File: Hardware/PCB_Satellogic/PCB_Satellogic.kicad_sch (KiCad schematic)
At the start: 4 parts, among them U1 E22-900M30S_LoRa, U2 Node-MCU_ESP32_38PINES, U3 TP4065_Modulo_cargador_de_bat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

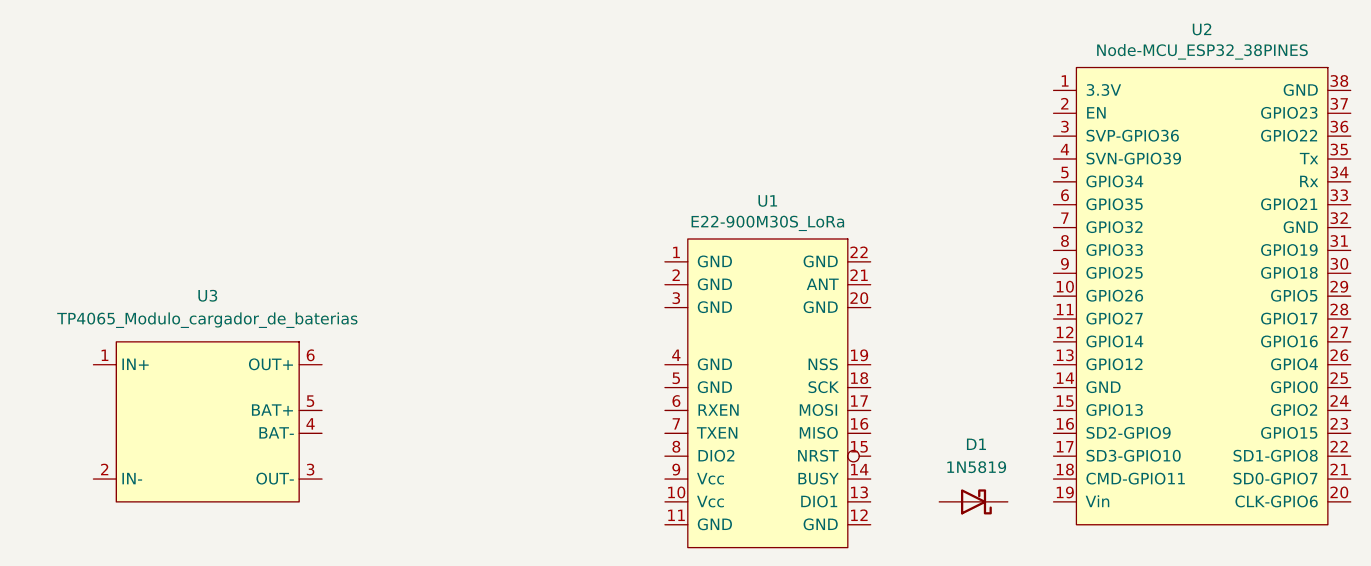
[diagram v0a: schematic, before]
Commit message: Introducción HW
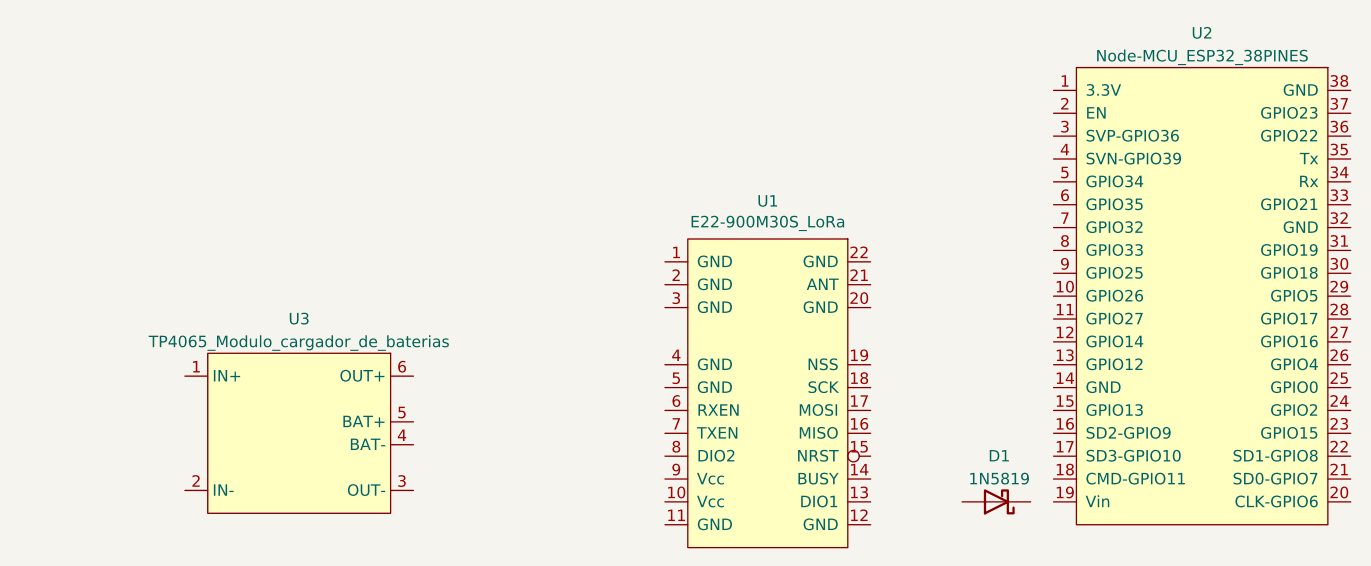
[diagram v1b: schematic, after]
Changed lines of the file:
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@@
-(kicad_sch (version 20211123) (generator eeschema)
+(kicad_sch (version 20230121) (generator eeschema)
   (paper "A4")
   (symbol (lib_id "Device:E22-900M30S_LoRa") (at 124.46 68.58 0) (unit 1)
-    (in_bom yes) (on_board yes)
-    (property "Reference" "U1" (id 0) (at 124.46 47.879 0))
-    (property "Value" "E22-900M30S_LoRa" (id 1) (at 124.46 50.1904 0))
-    (property "Footprint" "PCB_Satellogic:E22-900M30S_LoRa_smd" (id 2) (at 123.19 60.96 0)
+    (in_bom yes) (on_board yes) (dnp no)
+    (property "Reference" "U1" (at 124.46 47.879 0)
+      (effects (font (size 1.27 1.27)))
+    )
+    (property "Value" "E22-900M30S_LoRa" (at 124.46 50.1904 0)
+      (effects (font (size 1.27 1.27)))
+    )
+    (property "Footprint" "PCB_Satellogic:E22-900M30S_LoRa_smd" (at 123.19 60.96 0)
       (effects (font (size 1.27 1.27)) hide)
     )
-    (property "Datasheet" "" (id 3) (at 123.19 60.96 0)
+    (property "Datasheet" "" (at 123.19 60.96 0)
       (effects (font (size 1.27 1.27)) hide)
     )
@@
     (pin "8")
     (pin "9")
+    (instances
+      (project "PCB_Satellogic"
+        (path "/1c395ffa-f49b-425d-a435-d93dd675dfd0"
+          (reference "U1") (unit 1)
+        )
+      )
+    )
+  )
+  (symbol (lib_id "Diode:1N5819") (at 149.86 81.28 180) (unit 1)
+    (in_bom yes) (on_board yes) (dnp no) (fields_autoplaced)
+    (property "Reference" "D1" (at 150.1775 76.2 0)
+      (effects (font (size 1.27 1.27)))
+    )
+    (property "Value" "1N5819" (at 150.1775 78.74 0)
+      (effects (font (size 1.27 1.27)))
+    )
+    (property "Footprint" "Diode_THT:D_DO-41_SOD81_P10.16mm_Horizontal" (at 149.86 76.835 0)
+      (effects (font (size 1.27 1.27)) hide)
+    )
+    (property "Datasheet" "http://www.vishay.com/docs/88525/1n5817.pdf" (at 149.86 81.28 0)
+      (effects (font (size 1.27 1.27)) hide)
+    )
+    (pin "1")
+    (pin "2")
+    (instances
+      (project "PCB_Satellogic"
+        (path "/1c395ffa-f49b-425d-a435-d93dd675dfd0"
+          (reference "D1") (unit 1)
+        )
+      )
+    )
   )
   (symbol (lib_id "Device:Node-MCU_ESP32_38PINES") (at 172.72 57.15 0) (unit 1)
-    (in_bom yes) (on_board yes)
-    (property "Reference" "U2" (id 0) (at 172.72 28.829 0))
-    (property "Value" "Node-MCU_ESP32_38PINES" (id 1) (at 172.72 31.1404 0))
-    (property "Footprint" "PCB_Satellogic:Node-MCU_ESP32_38PINES_THT_offset" (id 2) (at 180.34 68.58 0)
+    (in_bom yes) (on_board yes) (dnp no) (fields_autoplaced)
+    (property "Reference" "U2" (at 172.72 29.21 0)
+      (effects (font (size 1.27 1.27)))
+    )
+    (property "Value" "Node-MCU_ESP32_38PINES" (at 172.72 31.75 0)
+      (effects (font (size 1.27 1.27)))
+    )
+    (property "Footprint" "PCB_Satellogic:Node-MCU_ESP32_38PINES_THT_offset" (at 180.34 68.58 0)
       (effects (font (size 1.27 1.27)) hide)
     )
-    (property "Datasheet" "" (id 3) (at 180.34 68.58 0)
+    (property "Datasheet" "" (at 180.34 68.58 0)
       (effects (font (size 1.27 1.27)) hide)
     )
@@
     (pin "8")
     (pin "9")
+    (instances
+      (project "PCB_Satellogic"
+        (path "/1c395ffa-f49b-425d-a435-d93dd675dfd0"
+          (reference "U2") (unit 1)
+        )
+      )
+    )
   )
-  (symbol (lib_id "Diode:1N5819") (at 147.32 81.28 180) (unit 1)
-    (in_bom yes) (on_board yes) (fields_autoplaced)
-    (property "Reference" "D1" (id 0) (at 147.6375 74.93 0))
-    (property "Value" "1N5819" (id 1) (at 147.6375 77.47 0))
-    (property "Footprint" "Diode_THT:D_DO-41_SOD81_P10.16mm_Horizontal" (id 2) (at 147.32 76.835 0)
+  (symbol (lib_id "Libreria_Proyecto_Satellogic:TP4065_Modulo_cargador_de_baterias") (at 72.39 73.66 0) (unit 1)
+    (in_bom yes) (on_board yes) (dnp no) (fields_autoplaced)
+    (property "Reference" "U3" (at 72.39 60.96 0)
+      (effects (font (size 1.27 1.27)))
+    )
+    (property "Value" "TP4065_Modulo_cargador_de_baterias" (at 72.39 63.5 0)
+      (effects (font (size 1.27 1.27)))
+    )
+    (property "Footprint" "PCB_Satellogic:TP4056" (at 71.12 68.58 0)
       (effects (font (size 1.27 1.27)) hide)
     )
-    (property "Datasheet" "http://www.vishay.com/docs/88525/1n5817.pdf" (id 3) (at 147.32 81.28 0)
-      (effects (font (size 1.27 1.27)) hide)
-    )
-    (pin "1")
-    (pin "2")
-  )
-  (symbol (lib_id "Libreria_Proyecto_Satellogic:TP4065_Modulo_cargador_de_baterias") (at 62.23 72.39 0) (unit 1)
-    (in_bom yes) (on_board yes) (fields_autoplaced)
-    (property "Reference" "U3" (id 0) (at 62.23 58.42 0))
-    (property "Value" "TP4065_Modulo_cargador_de_baterias" (id 1) (at 62.23 60.96 0))
-    (property "Footprint" "PCB_Satellogic:TP4056" (id 2) (at 60.96 67.31 0)
-      (effects (font (size 1.27 1.27)) hide)
-    )
-    (property "Datasheet" "" (id 3) (at 60.96 67.31 0)
+    (property "Datasheet" "" (at 71.12 68.58 0)
       (effects (font (size 1.27 1.27)) hide)
     )
@@
     (pin "5")
     (pin "6")
+    (instances
+      (project "PCB_Satellogic"
+        (path "/1c395ffa-f49b-425d-a435-d93dd675dfd0"
+          (reference "U3") (unit 1)
+        )
+      )
+    )
   )
   (sheet_instances
     (path "/" (page "1"))
   )
-  (symbol_instances
-    (path "/9dc25e6c-ccc6-4fa7-a0b9-7dc1baf8ff68"
-      (reference "D1") (unit 1) (value "1N5819") (footprint "Diode_THT:D_DO-41_SOD81_P10.16mm_Horizontal")
-    )
-    (path "/00000000-0000-0000-0000-0000640a4933"
-      (reference "U1") (unit 1) (value "E22-900M30S_LoRa") (footprint "PCB_Satellogic:E22-900M30S_LoRa_smd")
-    )
-    (path "/00000000-0000-0000-0000-0000640a5209"
-      (reference "U2") (unit 1) (value "Node-MCU_ESP32_38PINES") (footprint "PCB_Satellogic:Node-MCU_ESP32_38PINES_THT_offset")
-    )
-    (path "/db130f58-7442-4364-94e7-fd26116f26ed"
-      (reference "U3") (unit 1) (value "TP4065_Modulo_cargador_de_baterias") (footprint "PCB_Satellogic:TP4056")
-    )
-  )
 )
